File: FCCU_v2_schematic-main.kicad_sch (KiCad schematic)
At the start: 8 parts, among them J1 Supercapacitors, J2 CAN, J4 P_Valve, J5 FC_ON, J6 FC Module, J69 ADC, Freq, 4-20mA, J7 FC Cooling, J8 M_Valve

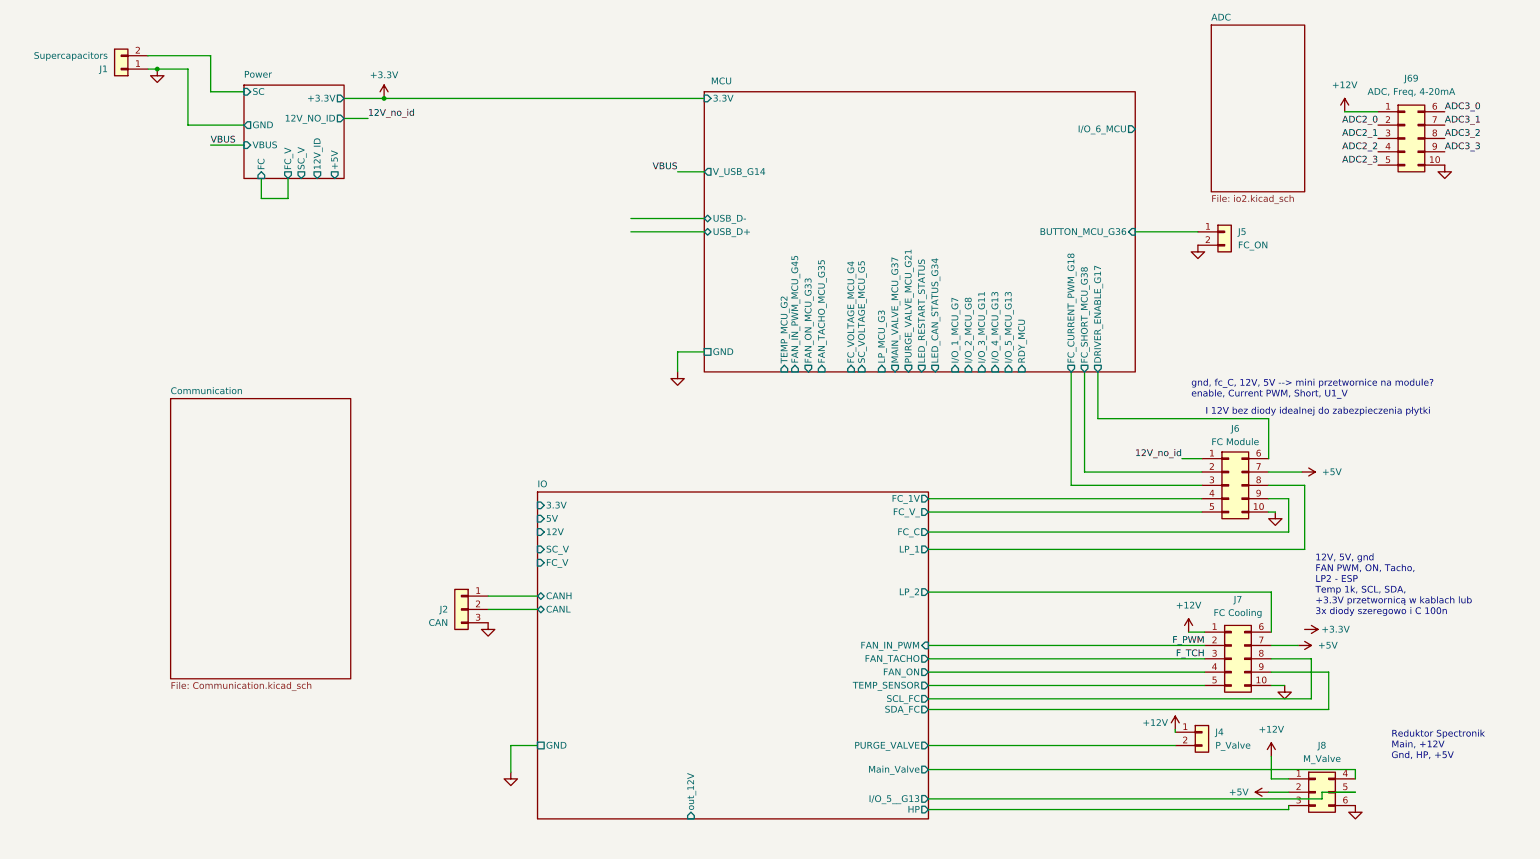
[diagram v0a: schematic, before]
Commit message: Full
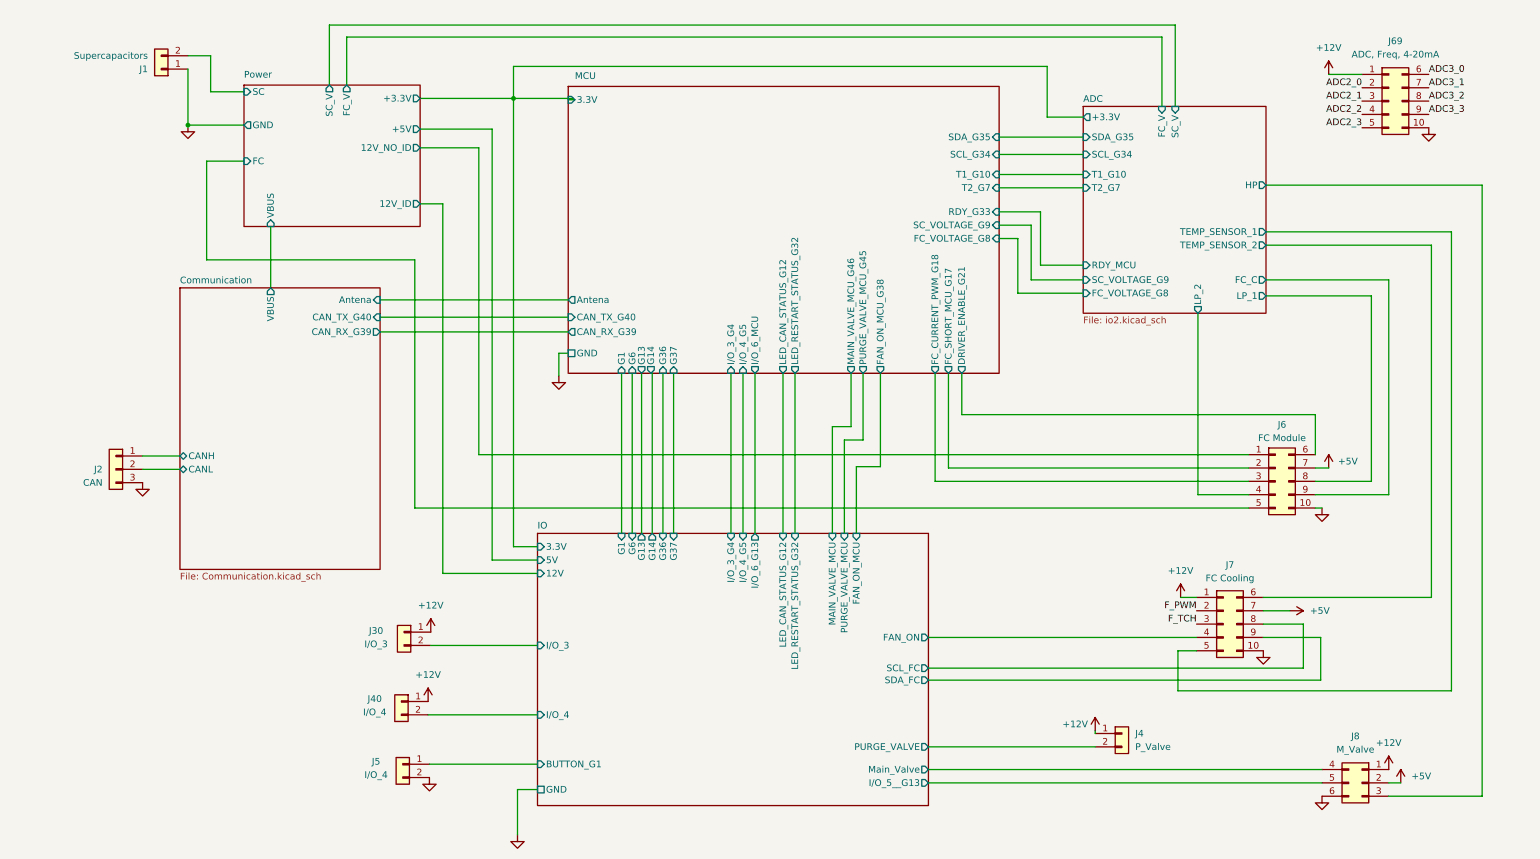
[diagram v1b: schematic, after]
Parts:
- added J30: I/O_3, Connector_Molex:Molex_Mini-Fit_Jr_5569-02A2_2x01_P4.20mm_Horizontal, symbol Connector_Generic:Conn_01x02
- added J5: I/O_4, Connector_Molex:Molex_Mini-Fit_Jr_5569-02A2_2x01_P4.20mm_Horizontal, symbol Connector_Generic:Conn_01x02
- J40: renamed from J5; value FC_ON -> I/O_4
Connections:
- net IO/FC_V_ is gone; now on net Power/FC: J6.5 (Pin_5)
- net MCU/BUTTON_MCU_G36 is gone; now on net +12V: J40.1 (Pin_1)
- net +12V: now also J30.1 (Pin_1)
- net GND: now also J5.2 (Pin_2); no longer J40.2 (Pin_2)
- net 12V_no_id renamed Power/12V_NO_ID
- net IO/CANH renamed Communication/CANH
- net IO/CANL renamed Communication/CANL
- net IO/FC_1V renamed ADC/LP_2
- net IO/FC_C renamed ADC/FC_C
- net IO/HP renamed ADC/HP
- net IO/LP_1 renamed ADC/LP_1
- net IO/LP_2 renamed ADC/TEMP_SENSOR_2
- net IO/TEMP_SENSOR renamed ADC/TEMP_SENSOR_1
- net MCU/DRIVER_ENABLE_G17 renamed MCU/DRIVER_ENABLE_G21
- net MCU/FC_SHORT_MCU_G38 renamed MCU/FC_SHORT_MCU_G17
- new net IO/BUTTON_G1: J5.1 (Pin_1)
- new net IO/I/O_3: J30.2 (Pin_2)
- new net IO/I/O_4: J40.2 (Pin_2)
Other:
- sheet ADC ports: added +3.3V, FC_C, FC_V, FC_VOLTAGE_G8, HP, LP_1, LP_2, RDY_MCU, SCL_G34, SC_V, SC_VOLTAGE_G9, SDA_G35, T1_G10, T2_G7, TEMP_SENSOR_1, TEMP_SENSOR_2; removed none
- sheet Communication ports: added Antena, CANH, CANL, CAN_RX_G39, CAN_TX_G40, VBUS; removed none
- sheet IO ports: added BUTTON_G1, FAN_ON_MCU, G1, G13, G14, G36, G37, G6, I/O_3, I/O_3_G4, I/O_4, I/O_4_G5, I/O_6_G13, LED_CAN_STATUS_G12, LED_RESTART_STATUS_G32, MAIN_VALVE_MCU, PURGE_VALVE_MCU; removed CANH, CANL, FAN_IN_PWM, FAN_TACHO, FC_1V, FC_C, FC_V, FC_V_, HP, LP_1, LP_2, SC_V, TEMP_SENSOR, out_12V
- sheet MCU ports: added Antena, CAN_RX_G39, CAN_TX_G40, DRIVER_ENABLE_G21, FAN_ON_MCU_G38, FC_SHORT_MCU_G17, FC_VOLTAGE_G8, G1, G13, G14, G36, G37, G6, I/O_3_G4, I/O_4_G5, LED_CAN_STATUS_G12, LED_RESTART_STATUS_G32, MAIN_VALVE_MCU_G46, PURGE_VALVE_MCU_G45, RDY_G33, SCL_G34, SC_VOLTAGE_G9, SDA_G35, T1_G10, T2_G7; removed BUTTON_MCU_G36, DRIVER_ENABLE_G17, FAN_IN_PWM_MCU_G45, FAN_ON_MCU_G33, FAN_TACHO_MCU_G35, FC_SHORT_MCU_G38, FC_VOLTAGE_MCU_G4, I/O_1_MCU_G7, I/O_2_MCU_G8, I/O_3_MCU_G11, I/O_4_MCU_G13, I/O_5_MCU_G13, LED_CAN_STATUS_G34, LED_RESTART_STATUS, LP_MCU_G3, MAIN_VALVE_MCU_G37, PURGE_VALVE_MCU_G21, RDY_MCU, SC_VOLTAGE_MCU_G5, TEMP_MCU_G2, USB_D+, USB_D-, V_USB_G14
- note removed: "12V, 5V, gnd FAN PWM, ON, Tacho, LP2 - ESP Temp 1k, SCL, SDA, +3.3V przetwornicą w kablach lub 3x diody szeregowo i C 100n"
- note removed: "I 12V bez diody idealnej do zabezpieczenia płytki"
- note removed: "Reduktor Spectronik Main, +12V Gnd, HP, +5V"
- note removed: "gnd, fc_C, 12V, 5V --> mini przetwornice na module? enable, Current PWM, Short, U1_V"
- moved on the sheet: J1, J2, J4, J40, J6, J69, J7
